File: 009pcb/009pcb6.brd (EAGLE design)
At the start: 160 x 100 mm, 35 parts

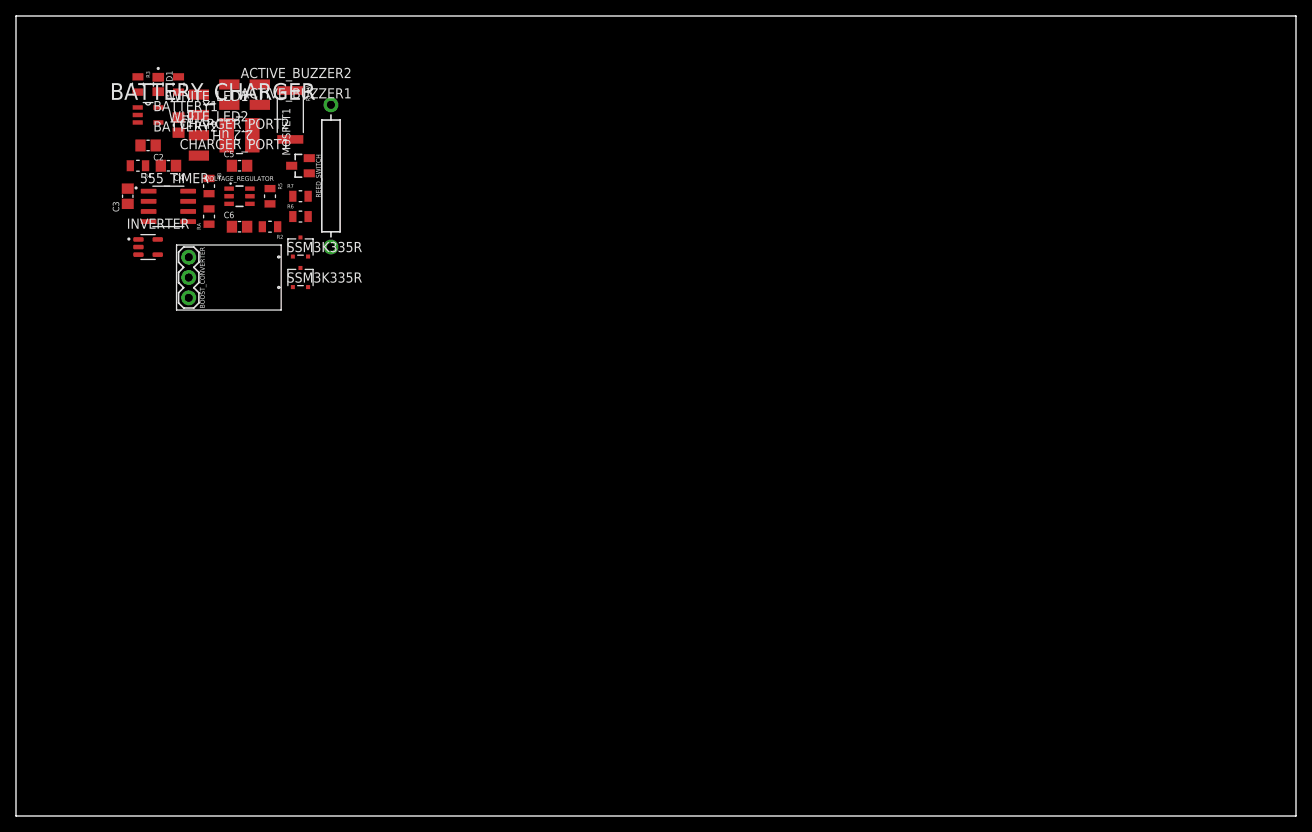
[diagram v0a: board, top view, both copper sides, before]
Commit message: sent for manufacturing
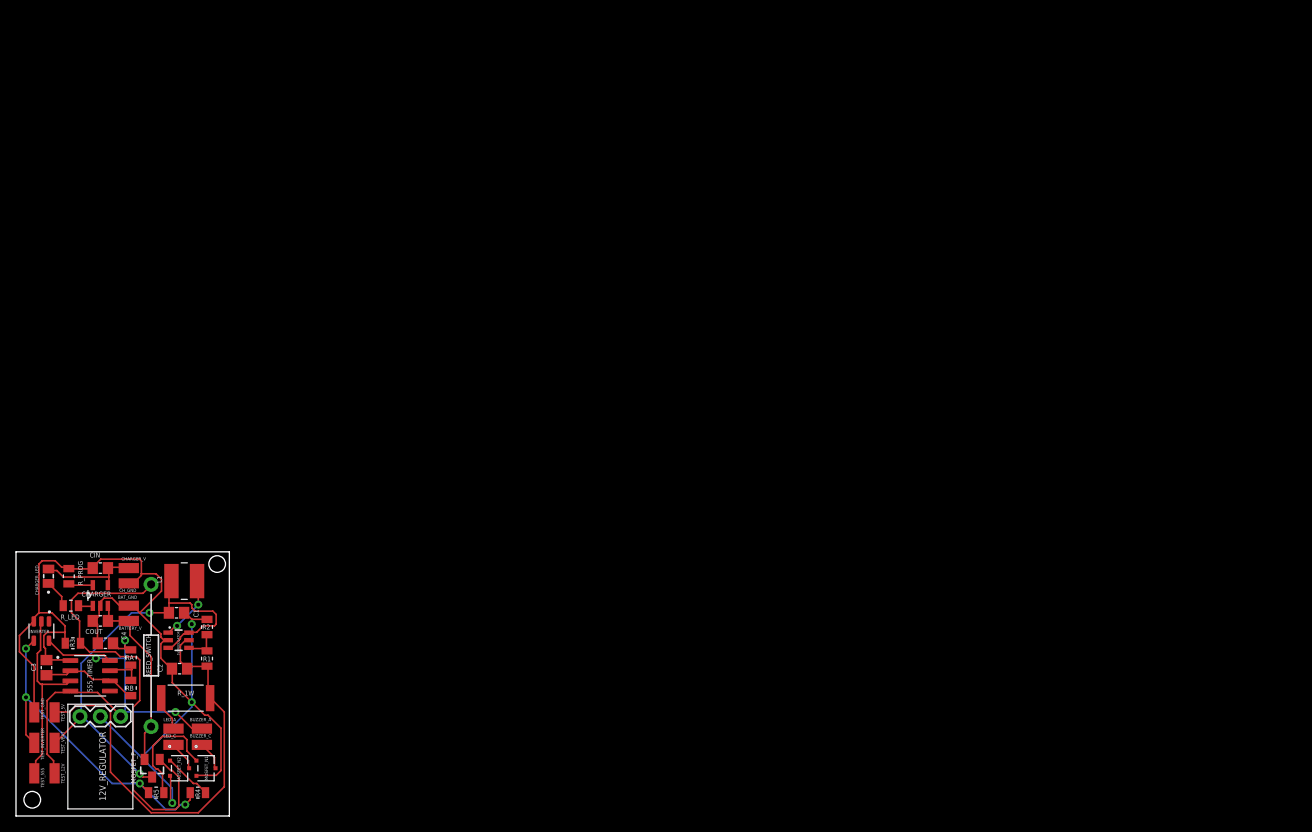
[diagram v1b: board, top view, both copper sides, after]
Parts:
- removed ACTIVE_BUZZER1, ACTIVE_BUZZER2, BATTERY1, BATTERY2, CHARGER_PORT1, CHARGER_PORT2, WHITE_LED1, WHITE_LED2: WIREPADSMD1,27-254, wirepad:SMD1,27-2,54
- removed BATTERY_CHARGER: MCP73831T-5ACI/OT, MCP73831T-5ACI_OT:SOT95P280X145-5N
- removed BOOST_CONVERTER: (no value), SparkFun-Connectors:1X03
- removed C5, C6: (no value), GRT21BR61H475ME13L:CAPC2012X135N
- removed D1: 5988170107F, 5988170107F:LEDC2012X70N
- removed MOSFET1: P_CHANNEL, DMP2004K:SOT23
- removed MOSFET2, MOSFET3: SSM3K335R, SSM3K335R:SOT-23F_TOS
- removed R1_1W: 4.7 Ω, RC2512FK-074R7L:RESC6331X65N
- removed R6, R7: 10 Ω, RC0805JR-0720KL:RESC2012X60N
- removed VOLTAGE_REGULATOR: TLV61070A, TLV61070A:SOT23-6
- added 12V_REGULATOR: (no value), SparkFun-Connectors:1X03
- added 5V_REGULATOR: (no value), TLV61070A:SOT23-6
- added BATTERY_V, BAT_GND, CHARGER_V, CH_GND, LED_A, LED_C, TEST_12V, TEST_555, TEST_5V, TEST_GND, TEST_INVERTER, TEST_VBAT: (no value), wirepad:SMD1,27-2,54
- added BUZZER_A, BUZZER_C: WIREPADSMD1,27-254, wirepad:SMD1,27-2,54
- added CHARGER: (no value), MCP73831T-5ACI_OT:SOT95P280X145-5N
- added CHARGER_LED: (no value), 5988170107F:LEDC2012X70N
- added CIN, COUT: 4.7 uF, GRT21BR61H475ME13L:CAPC2012X135N
- added MOSFET_N1, MOSFET_N2: (no value), SSM3K335R:SOT-23F_TOS
- added MOSFET_P: (no value), DMP2004K:SOT23
- added R_1W: 4.7 Ω, RC2512FK-074R7L:RESC6331X65N
- added R_LED: 220 Ω, RC0805JR-0720KL:RESC2012X60N
- added R_PROG: 10 kΩ, RC0805JR-0720KL:RESC2012X60N
- 555_TIMER: value NE555DR -> (none)
- C1, C2: value 4.7 uF -> (none)
- INVERTER: value BU4SU69G2-TR -> (none)
- R1: value 10 kΩ -> Ω
- R3: value 220 Ω -> 20 kΩ
- R4: value 20 kΩ -> 10 Ω
- R5: value Ω -> 10 Ω
- REED_SWITCH: value NORMALLY_OPEN -> (none); device SparkFun-Switches:REED_SWITCH_GLASS -> RI-80GP0510:REED_SWITCH_GLASS
- moved R4 78.7 mm to (22.7, 2.92), turned to 0 degrees
- moved R5 75.9 mm to (17.5, 2.92), turned to 0 degrees
- moved R1 71.8 mm to (23.9, 19.7), turned to 270 degrees
- moved R3 70.3 mm to (7.11, 21.6), turned to 180 degrees
- moved C2 65.5 mm to (20.4, 18.4)
- moved REED_SWITCH 64.0 mm to (16.9, 20.1), turned to 270 degrees
- moved RB 63.5 mm to (14.4, 16.0)
- moved C1 61.0 mm to (20.1, 25.4), turned to 0 degrees
- moved C4 60.2 mm to (11.2, 21.6)
- moved C3 59.8 mm to (3.81, 18.5)
- moved 555_TIMER 59.5 mm to (9.27, 17.5)
- moved L1 56.2 mm to (21.0, 29.4), turned to 0 degrees
- moved RA 56.0 mm to (14.4, 19.8)
- moved R2 50.7 mm to (23.9, 23.6), turned to 270 degrees
- moved INVERTER 49.8 mm to (3.17, 23.1), turned to 270 degrees
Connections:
- removed net VBAT1: C6.1
- net 12V: now also 12V_REGULATOR.1, BUZZER_A.1, TEST_12V.1; no longer ACTIVE_BUZZER1.1, BOOST_CONVERTER.1
- net 5V: now also 5V_REGULATOR.5, C2.1, R1.2, R_1W.2, TEST_5V.1; no longer R1_1W.2, R2.2, VOLTAGE_REGULATOR.5
- net GND: now also 12V_REGULATOR.2, 5V_REGULATOR.2, BAT_GND.1, CHARGER.2, CH_GND.1, CIN.2, COUT.2, MOSFET_N1.2, MOSFET_N2.2, R2.1, R3.2, R_PROG.1, TEST_GND.1; no longer BATTERY2.1, BATTERY_CHARGER.2, BOOST_CONVERTER.2, C5.2, C6.2, CHARGER_PORT2.1, MOSFET2.2, MOSFET3.2, R1.1, R4.2, R5.1, VOLTAGE_REGULATOR.2
- net N$10: now also 5V_REGULATOR.1; no longer VOLTAGE_REGULATOR.1
- net N$11: now also TEST_555.1
- net N$12: now also 5V_REGULATOR.4, R1.1, R2.2; no longer R2.1, R5.2, VOLTAGE_REGULATOR.4
- net N$13: now also R4.1, R5.1, TEST_INVERTER.1; no longer R6.1, R7.1
- net N$14: now also MOSFET_N2.1, R4.2; no longer MOSFET3.1, R7.2
- net N$15: now also LED_C.1, MOSFET_N2.3; no longer MOSFET3.3, WHITE_LED2.1
- net N$18: now also MOSFET_N1.1, R5.2; no longer MOSFET2.1, R6.2
- net N$19: now also BUZZER_C.1, MOSFET_N1.3; no longer ACTIVE_BUZZER2.1, MOSFET2.3
- net N$2: now also CHARGER.5, R_PROG.2; no longer BATTERY_CHARGER.5, R1.2
- net N$3: now also CHARGER_LED.C, R_LED.1; no longer D1.C, R3.1
- net N$4: now also MOSFET_P.1, R3.1; no longer MOSFET1.1, R4.1
- net N$5: now also CHARGER.1, R_LED.2; no longer BATTERY_CHARGER.1, R3.2
- net N$7: now also LED_A.1, R_1W.1; no longer R1_1W.1, WHITE_LED1.1
- net VBAT: now also BATTERY_V.1, CHARGER.3, COUT.1, MOSFET_P.2; no longer BATTERY1.1, BATTERY_CHARGER.3, C2.1, C5.1, L1.1, MOSFET1.2, VOLTAGE_REGULATOR.6
- net VCHARGE: now also CHARGER.4, CHARGER_LED.A, CHARGER_V.1, CIN.1; no longer BATTERY_CHARGER.4, C1.1, CHARGER_PORT1.1, D1.A
- net VIN: now also 12V_REGULATOR.3, 5V_REGULATOR.3, 5V_REGULATOR.6, C1.1, L1.1, MOSFET_P.3, TEST_VBAT.1; no longer BOOST_CONVERTER.3, MOSFET1.3, VOLTAGE_REGULATOR.3
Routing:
- net GND: track 0.00 -> 143.4 mm, vias 0 -> 3
- net 12V: track 0.00 -> 57.3 mm, vias 0 -> 3
- net VIN: track 0.00 -> 56.6 mm, vias 0 -> 2
- net 5V: track 0.00 -> 56.1 mm
- net N$4: track 0.00 -> 55.4 mm
- net N$13: track 0.00 -> 42.9 mm, vias 0 -> 4
- net N$11: track 0.00 -> 23.7 mm
- net VBAT: track 0.00 -> 23.5 mm
- net N$18: track 0.00 -> 14.6 mm
- net VCHARGE: track 0.00 -> 13.1 mm
- net N$6: track 0.00 -> 12.1 mm
- net N$10: track 0.00 -> 8.21 mm, vias 0 -> 2
- net N$14: track 0.00 -> 6.10 mm
- net N$8: track 0.00 -> 4.76 mm
- net N$7: track 0.00 -> 4.51 mm
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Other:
- board size 160 x 100 mm -> 26.7 x 33 mm
